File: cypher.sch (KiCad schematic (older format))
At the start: 30 parts, among them J2 AVR-ISP-6, J3 Breakout, Q1 MMBT3904, SW1 SW_Push, U1 ATmega32U4-MU, U2 PRTR5V0U2X, Y1 16Mhz

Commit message: cleanup of files - added bom in csv
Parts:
- J2: symbol Connector:AVR-ISP-6 -> cypher-rescue:AVR-ISP-6-Connector
- Q1: symbol transistors:MMBT3904 -> cypher-rescue:MMBT3904-transistors
- U1: symbol MCU_Microchip_ATmega:ATmega32U4-MU -> cypher-rescue:ATmega32U4-MU-MCU_Microchip_ATmega
- U2: symbol ai03-locallib:PRTR5V0U2X -> cypher-rescue:PRTR5V0U2X-ai03-locallib
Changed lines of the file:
@@
 	3665 6595 3940 6595
 $Comp
-L Connector:AVR-ISP-6 J2
+L cypher-rescue:AVR-ISP-6-Connector J2
 U 1 1 5C1571E9
 P 5815 2490
@@
 NoConn ~ 2090 1270
 $Comp
-L MCU_Microchip_ATmega:ATmega32U4-MU U1
+L cypher-rescue:ATmega32U4-MU-MCU_Microchip_ATmega U1
 U 1 1 5ED35339
 P 3065 5295
@@
 	3665 4295 3915 4295
 $Comp
-L ai03-locallib:PRTR5V0U2X U2
+L cypher-rescue:PRTR5V0U2X-ai03-locallib U2
 U 1 1 5D2FEB33
 P 3180 1510
@@
 	7935 1635 7935 1360
 $Comp
-L transistors:MMBT3904 Q1
+L cypher-rescue:MMBT3904-transistors Q1
 U 1 1 5E9E999A
 P 5390 4995

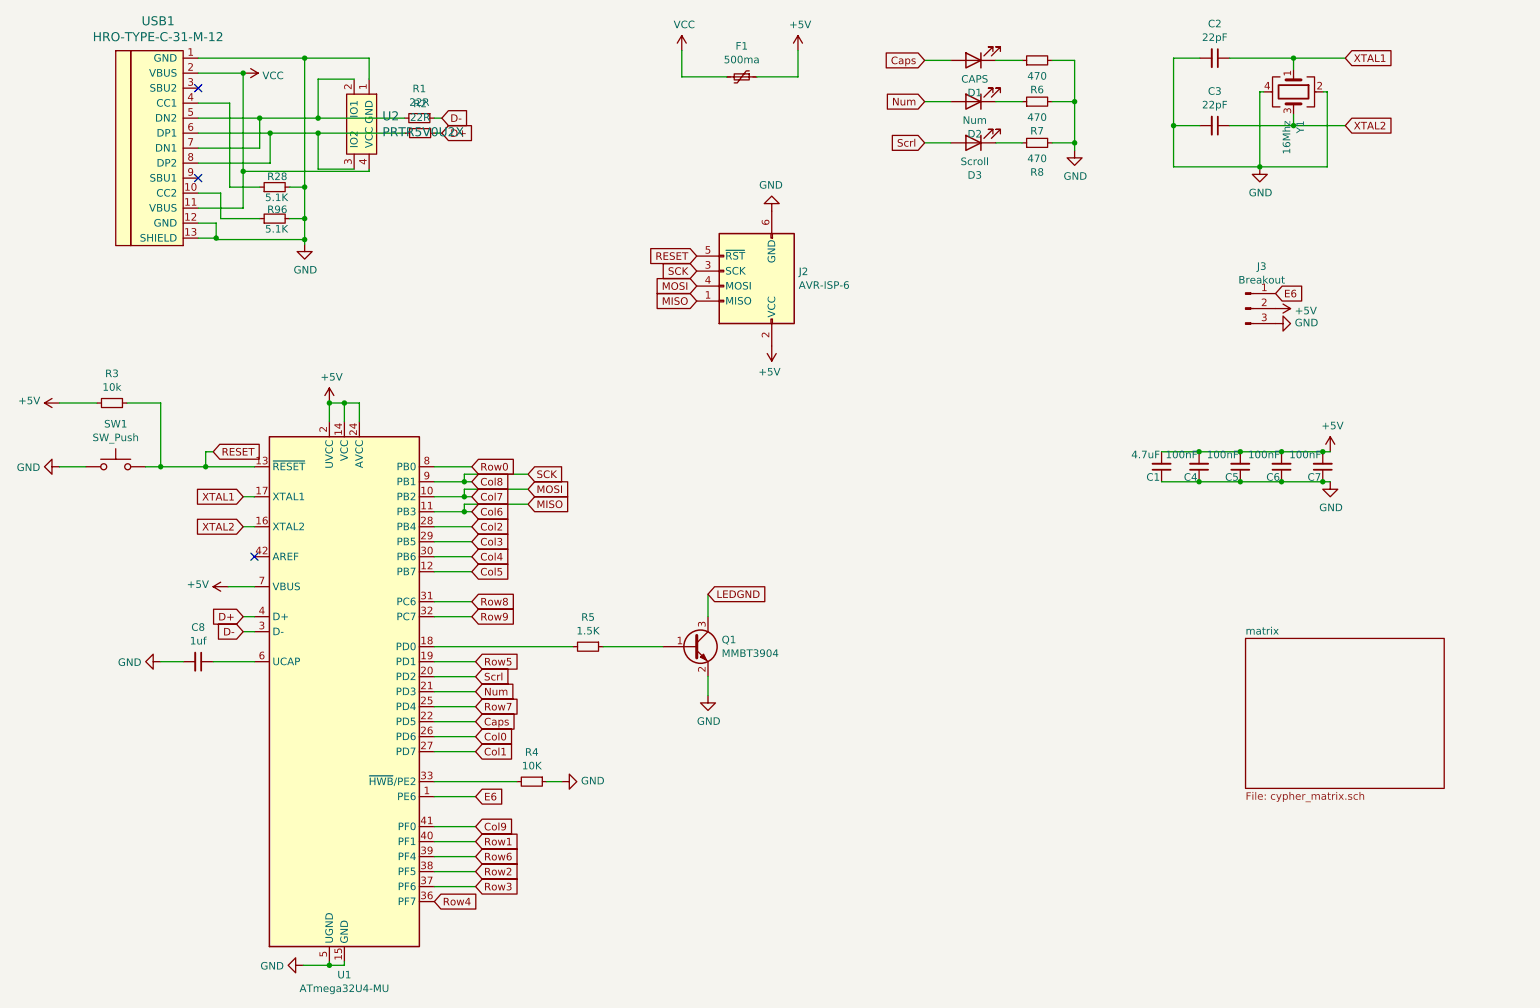
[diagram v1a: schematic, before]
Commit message: Cleanup and commit for rev6
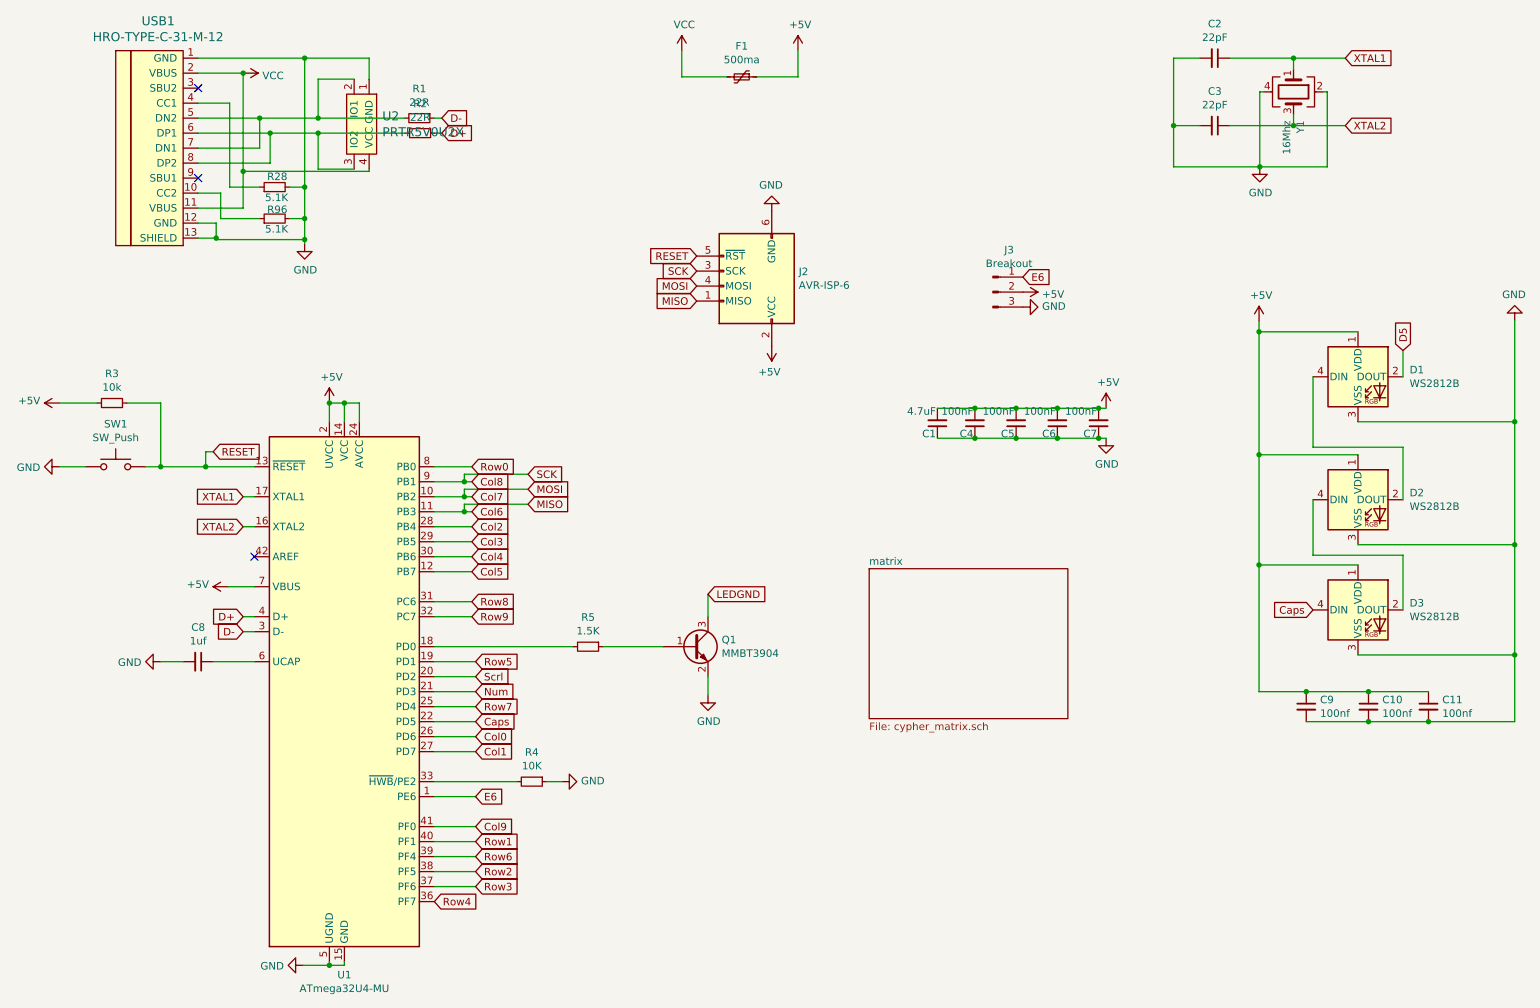
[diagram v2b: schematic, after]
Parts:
- removed D1: CAPS, LED_THT:LED_D1.8mm_W3.3mm_H2.4mm, symbol Device:LED
- removed D2: Num, LED_THT:LED_D1.8mm_W3.3mm_H2.4mm, symbol Device:LED
- removed D3: Scroll, LED_THT:LED_D1.8mm_W3.3mm_H2.4mm, symbol Device:LED
- removed R6, R7, R8: 470, Resistor_SMD:R_0603_1608Metric, symbol Device:R_Small
- added C10, C11, C9: 100nf, Capacitor_SMD:C_0603_1608Metric, symbol Device:C_Small
- added D1, D2, D3: WS2812B, CrumpPrints:WS2812-2020, symbol LED:WS2812B
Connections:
- net +5V: now also C10.1, C11.1, C9.1, D1.1 (VDD), D2.1 (VDD), D3.1 (VDD)
- net Caps: now also D3.4 (DIN)
- net GND: now also C10.2, C11.2, C9.2, D1.3 (VSS), D2.3 (VSS), D3.3 (VSS)
- new net: D1.4 (DIN), D2.2 (DOUT)
- new net: D2.4 (DIN), D3.2 (DOUT)
- new net D5: D1.2 (DOUT)
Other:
- moved on the sheet: C1, C4, C5, C6, C7, J3
